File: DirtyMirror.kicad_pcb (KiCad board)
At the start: 2 copper layers, 53 parts, among them J101 PWR, SW101 SW_SPDT, U101 TL074, U102 TL074, U103 TL072

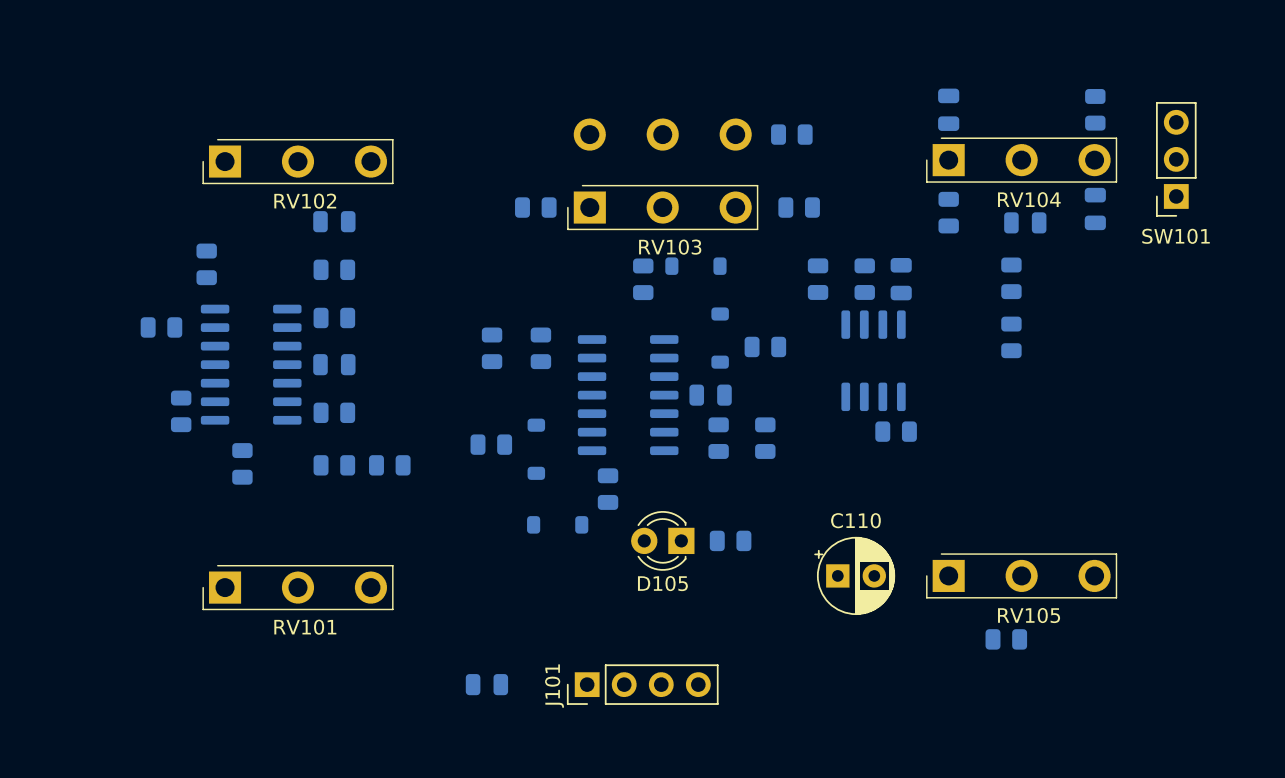
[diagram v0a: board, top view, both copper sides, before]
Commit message: routed & DRC passing
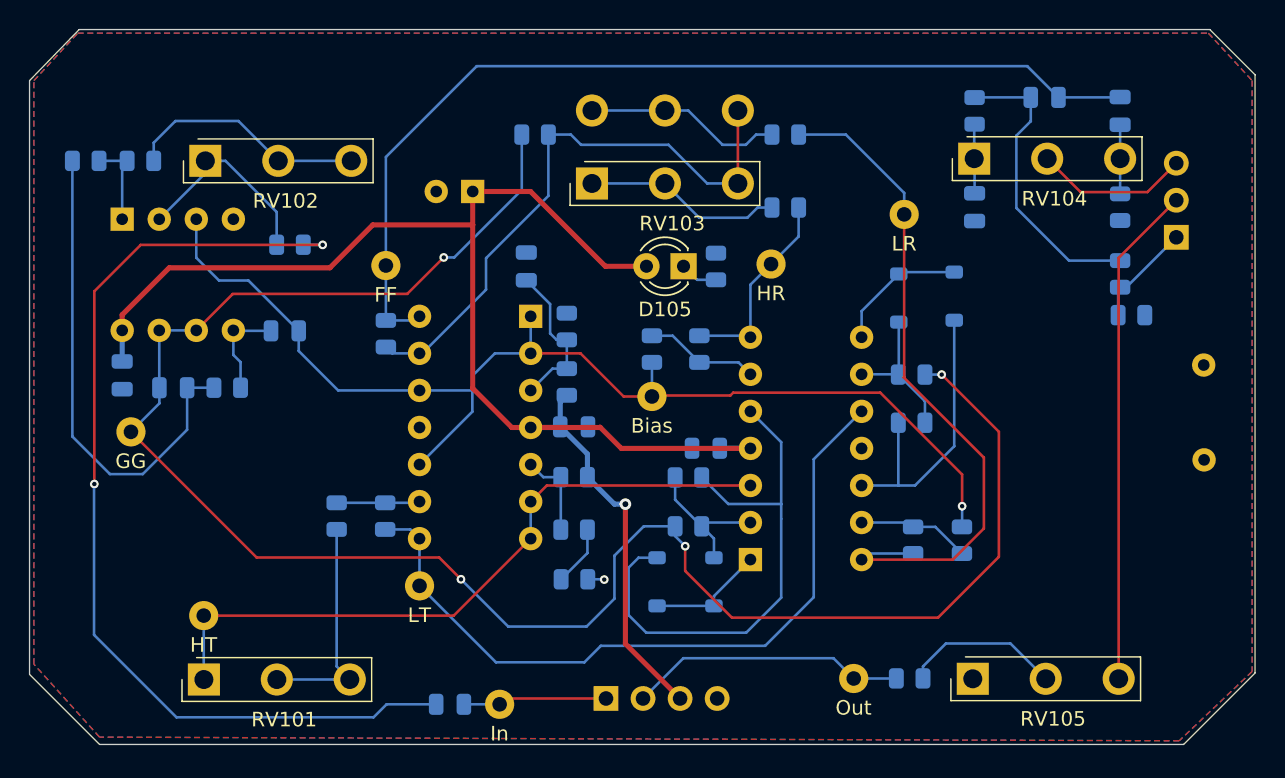
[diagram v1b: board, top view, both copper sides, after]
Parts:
- added C109: 4n7, Capacitor_SMD:C_0805_2012Metric, B.Cu at (21.7, 62.6)
- added C111: 2n2, Capacitor_SMD:C_0805_2012Metric, B.Cu at (14.1, 66.5)
- added J102: ScopeGroundLoop, Connector:THT_GND_WIRE, B.Cu at (84.7, 68.4)
- added TP101: In, TestPoint:TestPoint_THTPad_D2.0mm_Drill1.0mm_VAL, B.Cu at (36.4, 88.2)
- added TP102: Out, TestPoint:TestPoint_THTPad_D2.0mm_Drill1.0mm_VAL, B.Cu at (60.7, 86.5)
- added TP103: LT, TestPoint:TestPoint_THTPad_D2.0mm_Drill1.0mm_VAL, B.Cu at (30.9, 80.1)
- added TP104: HT, TestPoint:TestPoint_THTPad_D2.0mm_Drill1.0mm_VAL, B.Cu at (16.1, 82.2)
- added TP105: Bias, TestPoint:TestPoint_THTPad_D2.0mm_Drill1.0mm_VAL, B.Cu at (46.9, 67.2)
- added TP106: LR, TestPoint:TestPoint_THTPad_D2.0mm_Drill1.0mm_VAL, B.Cu at (64.2, 54.7)
- added TP107: HR, TestPoint:TestPoint_THTPad_D2.0mm_Drill1.0mm_VAL, B.Cu at (55.0, 58.1)
- added TP108: FF, TestPoint:TestPoint_THTPad_D2.0mm_Drill1.0mm_VAL, B.Cu at (28.6, 58.2)
- added TP109: GG, TestPoint:TestPoint_THTPad_D2.0mm_Drill1.0mm_VAL, B.Cu at (11.2, 69.6)
- C110, J101, SW101: moved to B.Cu
- R106, R107: value 47k -> 22k
- R123: value 100k -> 47k
- U101, U102: footprint Package_SO:SOIC-14_3.9x8.7mm_P1.27mm -> Package_DIP:DIP-14_W7.62mm
- U103: footprint Package_SO:SOIC-8_3.9x4.9mm_P1.27mm -> Package_DIP:DIP-8_W7.62mm
- moved C105 53.8 mm to (10.6, 65.7), turned to -90 degrees
- moved U103 52.4 mm to (10.6, 55.0), turned to -90 degrees
- moved R122 50.8 mm to (8.05, 51.0), turned to 180 degrees
- moved R123 44.3 mm to (17.8, 66.5), turned to 0 degrees
- moved C110 36.3 mm to (34.6, 53.1), turned to 180 degrees
- moved R121 35.6 mm to (28.6, 62.9), turned to 90 degrees
- moved R116 34.8 mm to (68.1, 77.0), turned to -90 degrees
- moved D104 31.4 mm to (67.6, 60.3), turned to 90 degrees
- moved R114 29.2 mm to (64.7, 65.7), turned to 180 degrees
- moved R117 28.7 mm to (64.8, 77.0), turned to -90 degrees
- moved D103 26.9 mm to (63.8, 60.4), turned to -90 degrees
- moved D102 21.8 mm to (47.2, 79.9), turned to 90 degrees
- moved R115 21.3 mm to (64.7, 69.0), turned to 180 degrees
- moved U101 19.4 mm to (38.5, 61.7)
- moved R129 18.8 mm to (51.2, 58.2), turned to 90 degrees
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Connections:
- R108 pad 2: /Gtr_Gain -> Net-(R108-Pad2)
- R109 pad 2: Net-(U101D--) -> Net-(U103A--)
- R111 pad 1: /Gtr_Gain -> /Gtr_gain
- R114 pad 1: /Gtr_Gain -> /Gtr_gain
- R120 pad 1: /Gtr_Gain -> /Gtr_gain
- R120 pad 2: Net-(U103A--) -> Net-(U101D--)
- R121 pad 1: Net-(U103A--) -> Net-(U101D--)
- R121 pad 2: Net-(R121-Pad2) -> /FxFull
- R122 pad 1: Net-(R121-Pad2) -> Net-(R108-Pad2)
- R122 pad 2: Net-(U103B--) -> Net-(C111-Pad1)
- R123 pad 1: Net-(U103B--) -> Net-(C111-Pad1)
- R123 pad 2: /FxFull -> Net-(U103B-+)
- RV102 pad 1: Net-(U101D--) -> Net-(U103A--)
- RV103 pad 1: Net-(U103A--) -> Net-(R118-Pad2)
- RV103 pad 2: Net-(U103A--) -> Net-(R118-Pad2)
- RV103 pad 3: Net-(R118-Pad2) -> Net-(U101D--)
- RV103 pad 4: Net-(U103A--) -> Net-(R119-Pad2)
- RV103 pad 5: Net-(U103A--) -> Net-(R119-Pad2)
- RV103 pad 6: Net-(R119-Pad2) -> Net-(U101D--)
- U101 pad 14: /Gtr_Gain -> /FxFull
- U103 pad 1: Net-(R121-Pad2) -> Net-(R108-Pad2)
- U103 pad 5: /Bias -> Net-(U103B-+)
- U103 pad 6: Net-(U103B--) -> /Gtr_gain
- U103 pad 7: /FxFull -> /Gtr_gain
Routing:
- net /Gtr_gain: track 0.00 -> 131.0 mm, vias 0 -> 4
- net +9V: track 0.00 -> 107.0 mm, vias 0 -> 1
- net /Bias: track 0.00 -> 80.0 mm, vias 0 -> 1
- net Net-(C103-Pad2): track 0.00 -> 68.0 mm, vias 0 -> 2
- net /FxFull: track 0.00 -> 67.4 mm
- net /LoThresh: track 0.00 -> 51.0 mm
- net /LoRect: track 0.00 -> 47.1 mm
- net /HiThresh: track 0.00 -> 47.0 mm
- net Net-(U101D--): track 0.00 -> 40.6 mm
- net Net-(D102-A): track 0.00 -> 37.3 mm
- net Net-(SW101-B): track 0.00 -> 34.4 mm
- net Net-(C111-Pad1): track 0.00 -> 33.8 mm
- net Net-(C106-Pad2): track 0.00 -> 20.5 mm
- net Net-(D104-K): track 0.00 -> 20.4 mm
- net FX_OUT: track 0.00 -> 19.1 mm
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- added copper zone on B.Cu, net GND
- added copper zone on F.Cu, net GND
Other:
- board outline added: 84 x 49 mm
- board text added: "+9V"
- board text added: "GND"
- board text added: "IN"
- board text added: "OUT"
